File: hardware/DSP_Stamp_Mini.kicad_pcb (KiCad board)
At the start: 2 copper layers, 37.5 x 62 mm, 73 parts, among them J1 Conn_01x10, J2 SM03B-SRSS-TB, J3 Conn_01x05, J4 USB_C_Receptacle_USB2.0_14P, J6 Conn_01x10, J7 Conn_01x02, J8 Conn_01x04, SW1 SW_Push, SW2 SW_Push, U1 RP2350_80QFN, U2 PCM3060, U3 DNF, U4 W25Q128JVS, U6 AZ1117-3.3, Y1 ABM8-272-T3

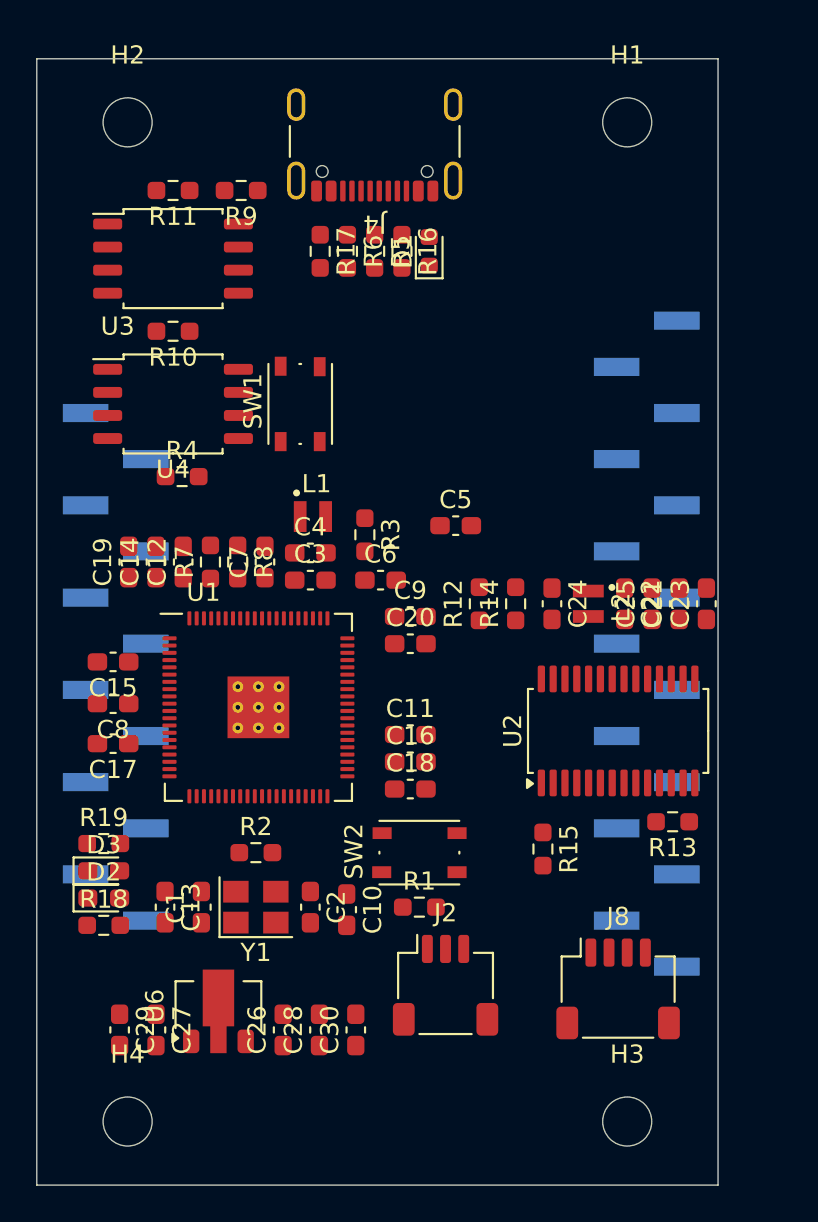
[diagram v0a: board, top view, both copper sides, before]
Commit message: repo cleanup
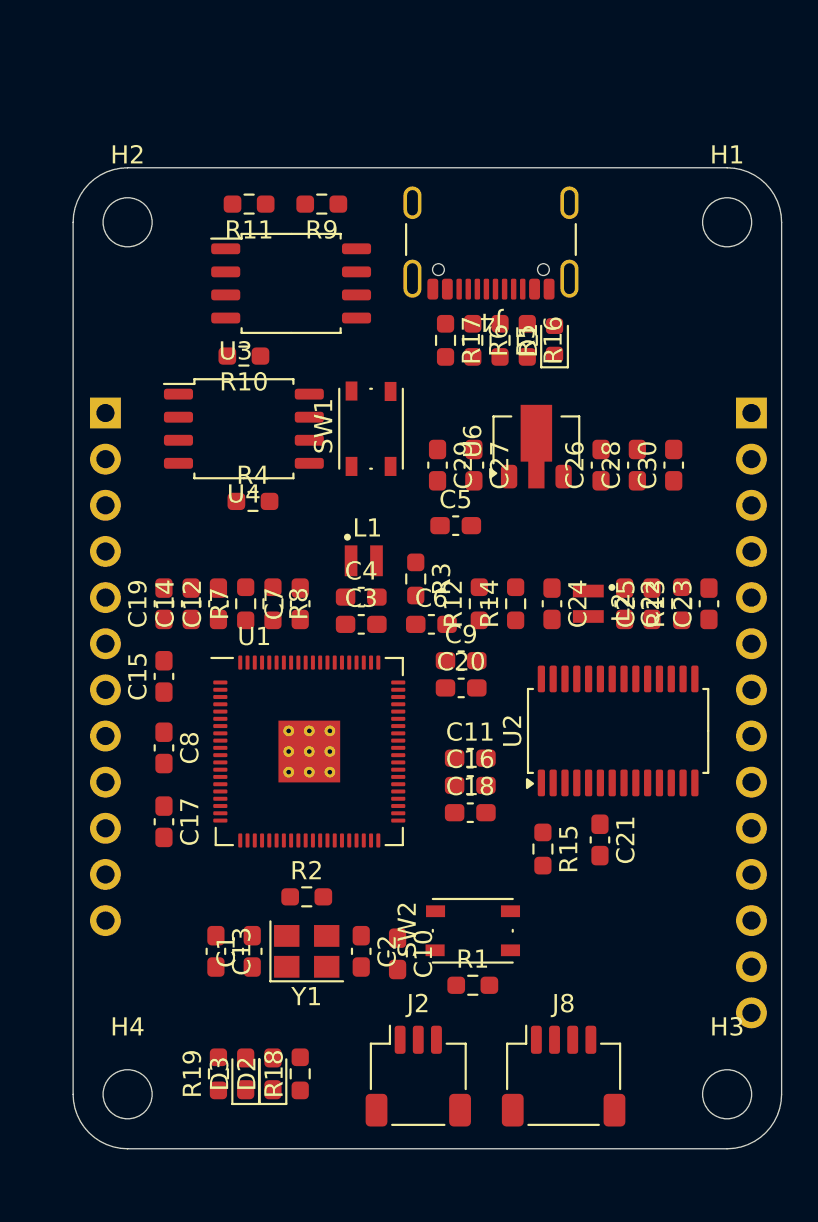
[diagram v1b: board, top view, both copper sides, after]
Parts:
- removed J3: Conn_01x05, Connector_PinHeader_2.54mm:PinHeader_1x05_P2.54mm_Vertical_SMD_Pin1Right
- removed J6: Conn_01x10, Connector_PinHeader_2.54mm:PinHeader_1x10_P2.54mm_Vertical_SMD_Pin1Right
- removed J7: Conn_01x02, Connector_PinHeader_2.54mm:PinHeader_1x02_P2.54mm_Vertical_SMD_Pin1Right
- added J5: Conn_01x12, Connector_PinHeader_2.54mm:PinHeader_1x12_P2.54mm_Vertical, B.Cu at (93.8, 63.5)
- J1: value Conn_01x10 -> Conn_01x14; footprint Connector_PinHeader_2.54mm:PinHeader_1x10_P2.54mm_Vertical_SMD_Pin1Right -> Connector_PinHeader_2.54mm:PinHeader_1x14_P2.54mm_Vertical
- moved U6 35.7 mm to (117.5, 65.0)
- moved C26 35.7 mm to (121.1, 66.4)
- moved C27 35.7 mm to (114.1, 66.4)
- moved C28 35.7 mm to (123.1, 66.4)
- moved C29 35.7 mm to (112.1, 66.4)
- moved C30 35.7 mm to (125.1, 66.4)
- moved J1 19.9 mm to (129.3, 63.5), turned to 180 degrees
- moved R19 14.2 mm to (100.0, 99.9), turned to 90 degrees
- moved C21 13.7 mm to (121.0, 87.0), turned to -90 degrees
- moved D3 13.6 mm to (101.5, 99.9), turned to 90 degrees
- moved R18 13.6 mm to (104.5, 99.9), turned to 90 degrees
- moved D2 13.4 mm to (103.0, 99.9), turned to 90 degrees
- moved R13 12.0 mm to (125.5, 74.0), turned to 90 degrees
- moved D1 8.46 mm to (118.5, 59.5)
- moved R16 8.46 mm to (117.0, 59.5)
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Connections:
- J1 pad 2: /GPIO40_ADC0 -> /GPIO47_ADC7
- J1 pad 3: /GPIO41_ADC1 -> /GPIO46_ADC6
- J1 pad 4: /GPIO42_ADC2 -> /GPIO45_ADC5
- J1 pad 5: /GPIO43_ADC3 -> /GPIO44_ADC4
- J1 pad 6: /GPIO44_ADC4 -> /GPIO43_ADC3
- J1 pad 7: /GPIO45_ADC5 -> /GPIO42_ADC2
- J1 pad 8: /GPIO46_ADC6 -> /GPIO41_ADC1
- J1 pad 9: /GPIO47_ADC7 -> /GPIO40_ADC0
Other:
- board size 37.5 x 62 mm -> 39 x 54 mm
